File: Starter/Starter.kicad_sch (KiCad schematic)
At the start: 50 parts, among them J2 Speaker, J3 UART1, J5 Conn_01x08_Pin, J7 DACOUT, SW1 UP, SW2 LEFT, SW3 DOWN, SW4 RIGHT, U2 LP-MSPM0G3507, U3 MCP34119P, U4 HiLetGo_ST7735R, U5 ULN2003B, U6 TSOP31438

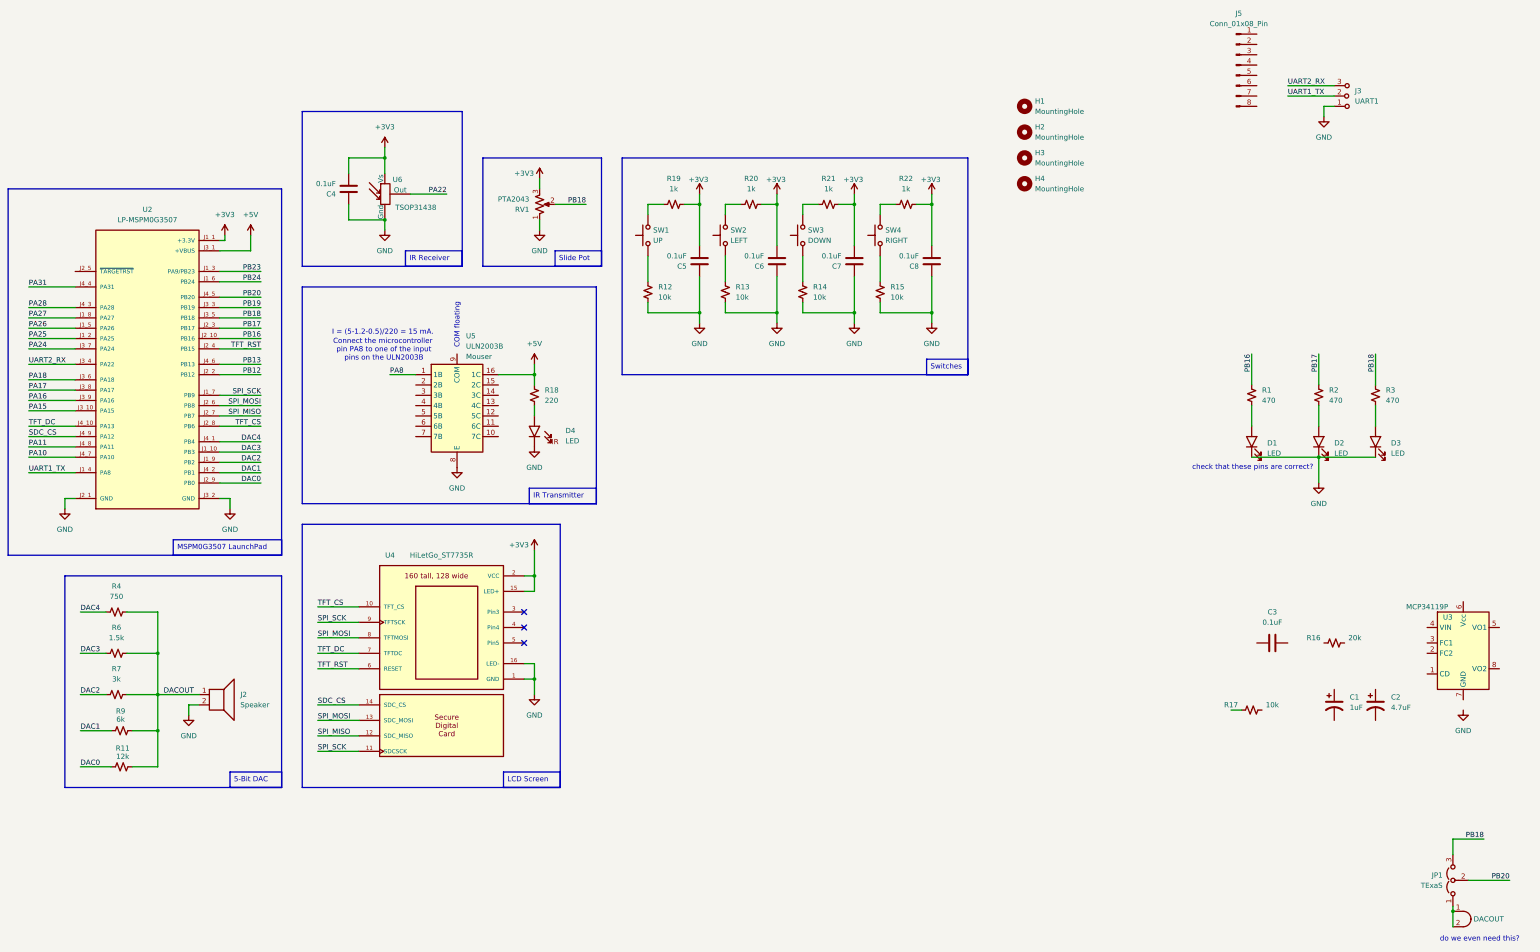
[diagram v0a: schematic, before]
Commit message: speaker amp
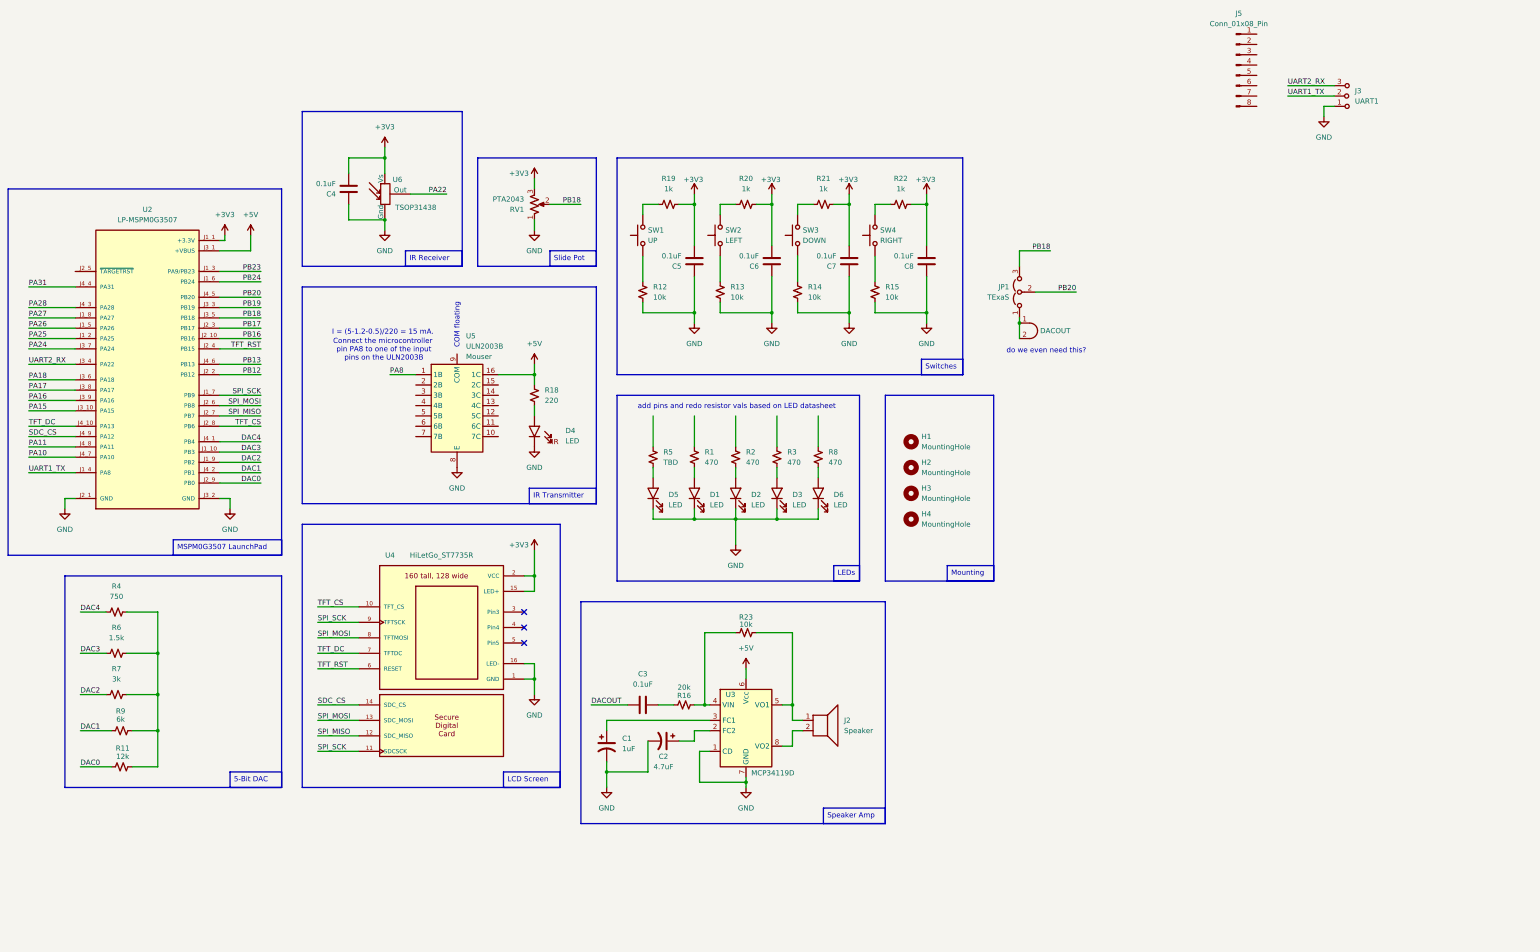
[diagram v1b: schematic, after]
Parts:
- removed R17: 10k, ECE319K:R_Axial_DIN0204_L3.6mm_D1.6mm_P7.62mm_Horizontal, symbol ECE319K:R_0.125W
- added D5, D6: LED, ECE319K:LED_D5.0mm, symbol ECE319K:LED
- added R23: 10k, ECE319K:R_Axial_DIN0204_L3.6mm_D1.6mm_P7.62mm_Horizontal, symbol ECE319K:R_0.125W
- added R5: TBD, ECE319K:R_Axial_DIN0204_L3.6mm_D1.6mm_P7.62mm_Horizontal, symbol ECE319K:R_0.125W
- added R8: 470, ECE319K:R_Axial_DIN0204_L3.6mm_D1.6mm_P7.62mm_Horizontal, symbol ECE319K:R_0.125W
- U3: value MCP34119P -> MCP34119D
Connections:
- net +5V: now also U3.6 (Vcc)
- net DACOUT: now also C3.1; no longer J2.1, R11.1, R4.1, R6.1, R7.1, R9.1
- net GND: now also C1.2, C2.2, U3.1 (CD), U3.7 (GND), D5.1 (K), D6.1 (K); no longer J2.2
- net PB16: no longer R1.1
- net PB17: no longer R2.1
- net PB18: no longer R3.1
- net at U3.2 (FC2): now also C2.1
- net at U3.3 (FC1): now also C1.1
- net at U3.4 (VIN): now also R16.1, R23.2
- net at U3.5 (VO1): now also J2.1, R23.1
- net at U3.8 (VO2): now also J2.2
- net at R16.2: now also C3.2
- new net: R11.1, R4.1, R6.1, R7.1, R9.1
- new net: D6.2 (A), R8.2
- new net: D5.2 (A), R5.2
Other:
- note added: "add pins and redo resistor vals based on LED datasheet"
- note removed: "check that these pins are correct?"
- moved on the sheet: C1, C2, C3, C5, C6, C7, C8, D1, D2, D3, H1, H2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
